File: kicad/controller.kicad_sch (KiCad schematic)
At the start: 38 parts, among them M5 Motor_DC, M6 Motor_DC, M7 Motor_DC, M8 Motor_DC, U10 DRV8833PW, U6 ESP32-DEVKITC, U8 GY-521

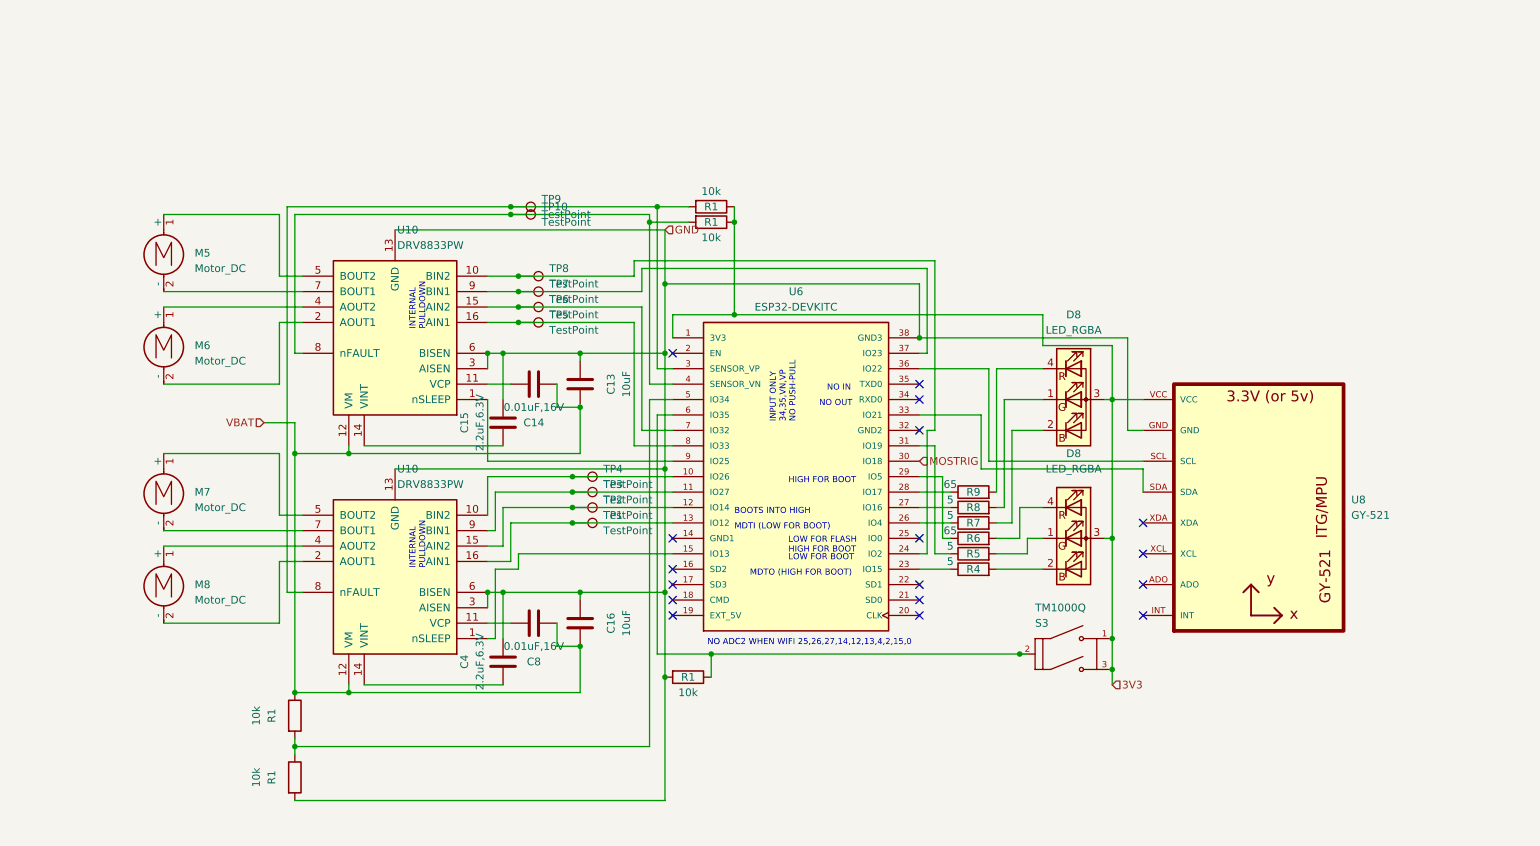
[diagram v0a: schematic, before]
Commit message: Make schematic pretty
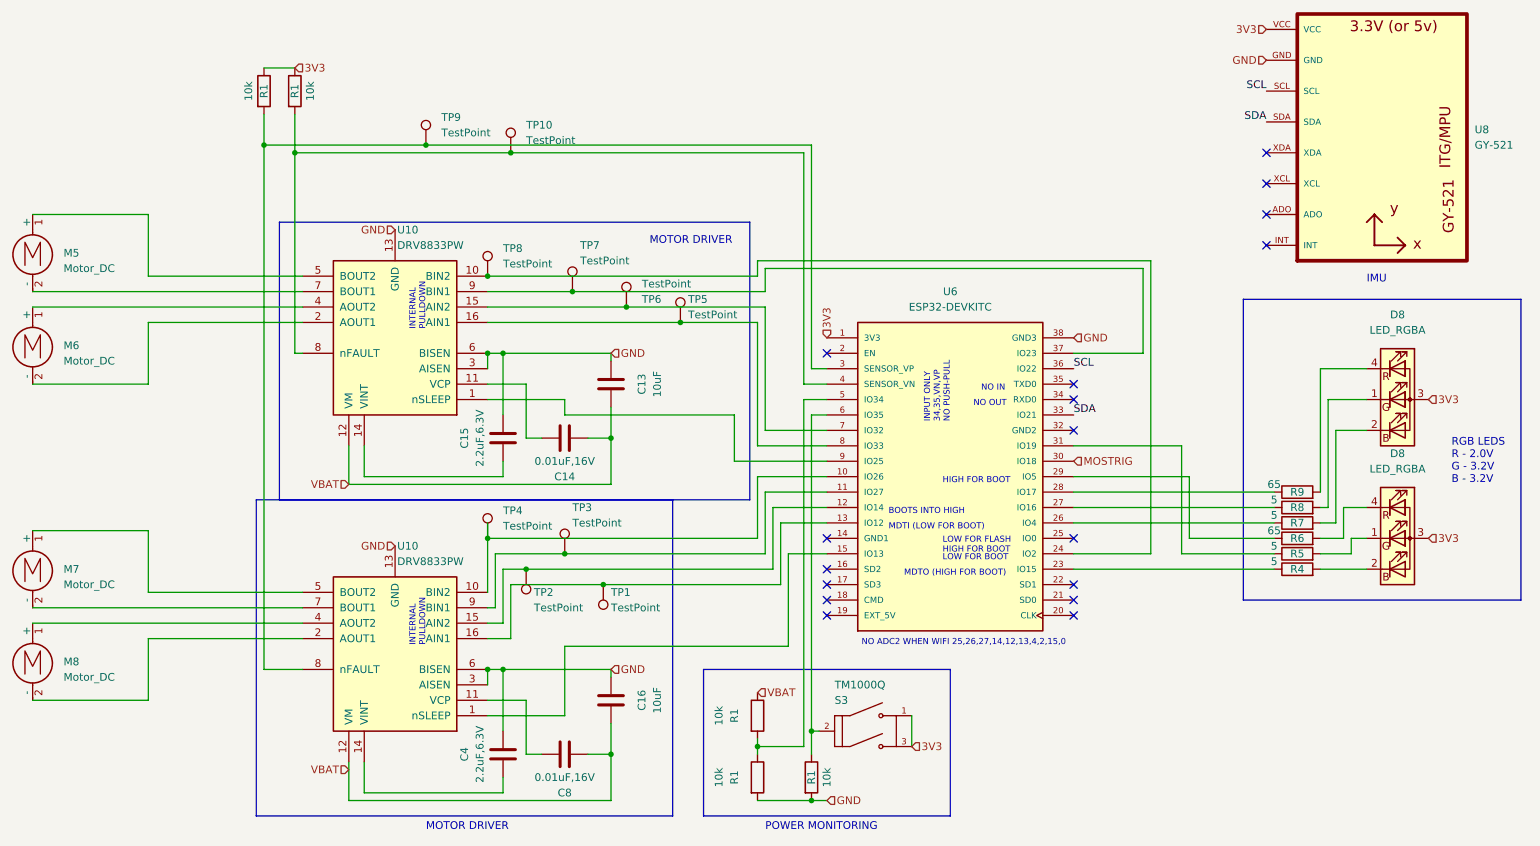
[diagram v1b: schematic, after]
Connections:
- net SCL: now reaches U6.36 (IO22), U8.SCL
- net SDA: now reaches U6.33 (IO21), U8.SDA
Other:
- note added: "IMU"
- note added: "MOTOR DRIVER"
- note added: "POWER MONITORING"
- note added: "RGB LEDS R - 2.0V G - 3.2V B - 3.2V"
- moved on the sheet: C13, C14, C15, C16, C4, C8, D8, M5, M6, M7, M8, R1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
